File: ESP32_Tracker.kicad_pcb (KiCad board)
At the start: 4 copper layers, 45.5 x 75.5 mm, 73 parts, among them J1 USB_C_Receptacle_USB2.0_16P, J2 Conn_01x02_Socket, J3 Conn_01x07_Socket, J4 MSD-4-A, SW1 SW_Push, SW2 SW_Push, SW3 SW_Push, SW4 SW_Push, SW5 SW_Push, U1 USBLC6-2SC6, U2 ESP32-S3-MINI-1, U3 MP2667, U4 XC6220B331MR-G, U5 LIS2MDL, U6 SAM-M10Q

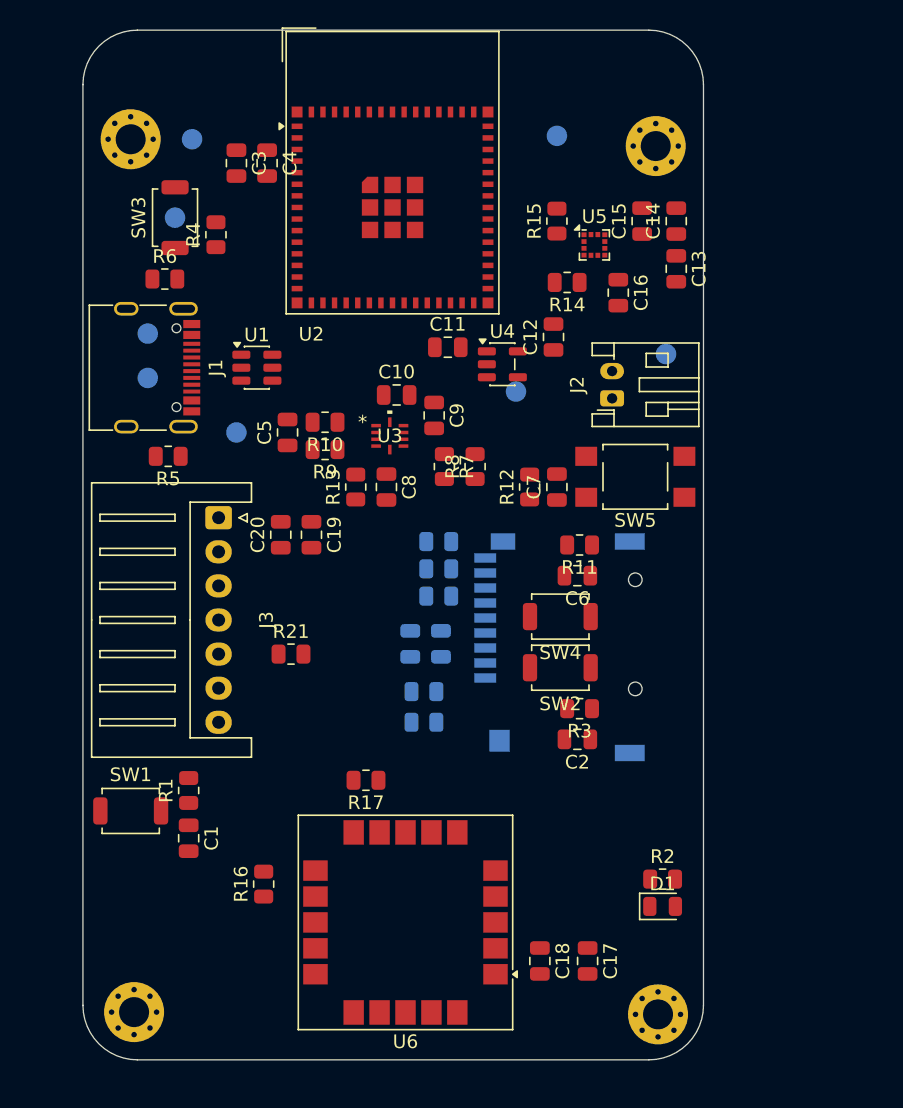
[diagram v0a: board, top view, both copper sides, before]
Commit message: Layout completed
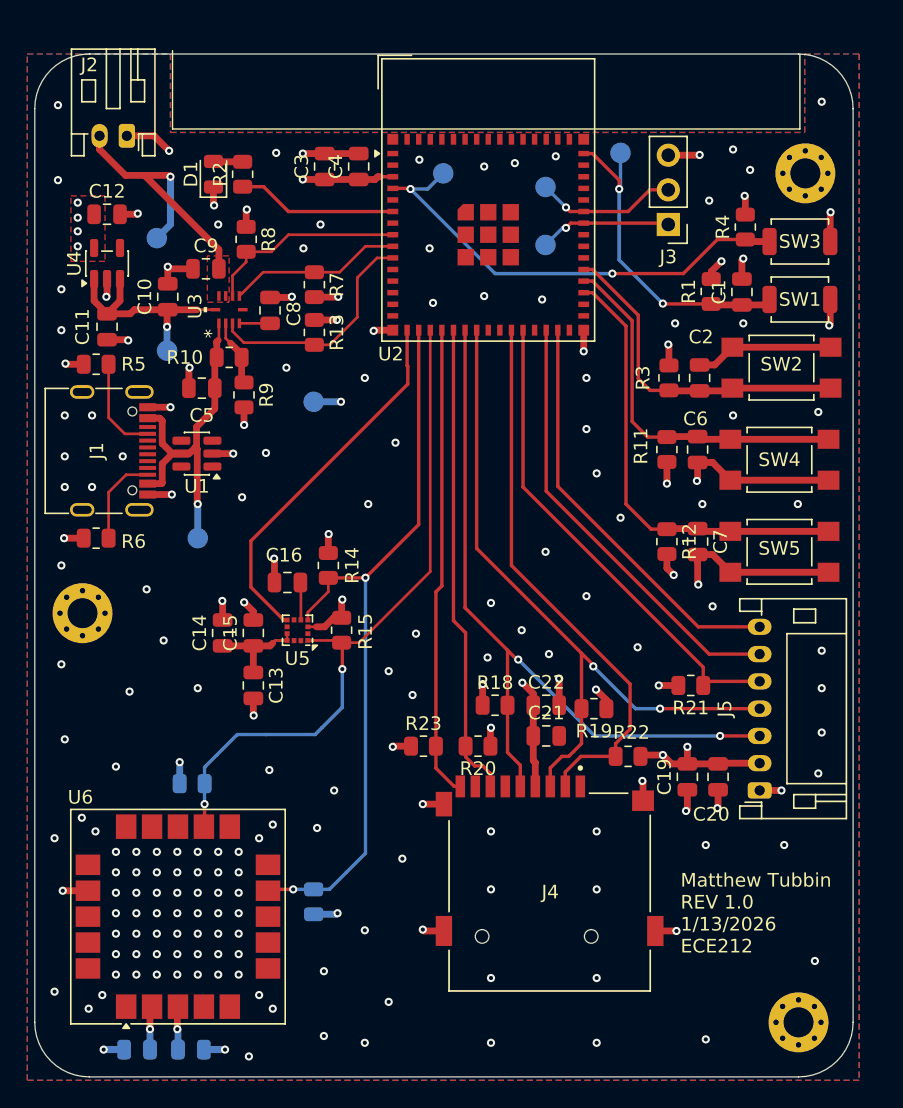
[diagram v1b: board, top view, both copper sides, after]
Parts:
- removed H4: MountingHole_Pad, MountingHole:MountingHole_2.2mm_M2_Pad_Via
- added J5: Conn_01x07_Socket, Connector_JST:JST_PH_S7B-PH-K_1x07_P2.00mm_Horizontal, F.Cu at (167.2, 116.0)
- C17: value 2.2u -> 10u; moved to B.Cu
- C18, R16, R17: moved to B.Cu
- C21, C22, J4, R18, R19, R20, R22, R23: moved to F.Cu
- J3: value Conn_01x07_Socket -> Conn_01x03; footprint Connector_JST:JST_XH_S7B-XH-A_1x07_P2.50mm_Horizontal -> Connector_PinHeader_2.54mm:PinHeader_1x03_P2.54mm_Vertical
- SW2, SW4: footprint Button_Switch_SMD:SW_SPST_TS-1088-xR020 -> Button_Switch_SMD:SW_SPST_TL3305C
- moved H2 81.2 mm to (170.1, 133.0)
- moved D1 63.0 mm to (127.2, 70.8), turned to 90 degrees
- moved SW1 61.8 mm to (170.2, 80.0), turned to 180 degrees
- moved R2 60.2 mm to (129.3, 70.8), turned to 90 degrees
- moved C1 57.0 mm to (165.9, 79.5), turned to 90 degrees
- moved R1 53.0 mm to (163.7, 79.4)
- moved SW3 45.8 mm to (170.2, 75.8), turned to 0 degrees
- moved C14 44.9 mm to (127.8, 104.5)
- moved C13 43.5 mm to (130.1, 108.3)
- moved C15 41.5 mm to (130.1, 104.5)
- moved J2 40.5 mm to (120.8, 68.0), turned to 180 degrees
- moved J3 39.4 mm to (160.5, 74.5), turned to 180 degrees
- moved R4 38.8 mm to (166.2, 74.7)
- moved TP6 38.3 mm to (123.0, 75.5)
- moved C20 36.6 mm to (164.2, 115.0), turned to -90 degrees
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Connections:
- net Net-(J2-Pin_2) renamed +BATT
- C2 pad 1: Net-(U2-IO18) -> /MCU/PWR/SW_TOGGLE
- C6 pad 1: Net-(U2-IO42) -> /MCU/PWR/SW_PWR
- C7 pad 1: Net-(U2-IO21) -> /MCU/PWR/SW_LOG
- J1 pad A6: Net-(J1-D+-PadA6) -> unconnected-(J1-D+-PadA6)
- J1 pad A7: Net-(J1-D--PadA7) -> unconnected-(J1-D--PadA7)
- J1 pad B6: Net-(J1-D+-PadA6) -> unconnected-(J1-D+-PadB6)
- J1 pad B7: Net-(J1-D--PadA7) -> unconnected-(J1-D--PadB7)
- J3 pad 1: GND -> /MCU/PWR/TX
- J3 pad 2: +3.3V -> /MCU/PWR/RX
- J3 pad 3: /MCU/PWR/OLED/SD_SCK -> GND
- R11 pad 1: Net-(U2-IO42) -> /MCU/PWR/SW_PWR
- R12 pad 1: Net-(U2-IO21) -> /MCU/PWR/SW_LOG
- R13 pad 2: /MCU/PWR/INT -> /MCU/PWR/BATT_INT
- R2 pad 1: Net-(U2-IO8) -> Net-(U2-IO2)
- R3 pad 1: Net-(U2-IO18) -> /MCU/PWR/SW_TOGGLE
- SW2 pad 1: Net-(U2-IO18) -> GND
- SW2 pad 2: GND -> /MCU/PWR/SW_TOGGLE
- SW4 pad 1: Net-(U2-IO42) -> /MCU/PWR/SW_PWR
- SW5 pad 1: Net-(U2-IO21) -> /MCU/PWR/SW_LOG
- TP2 pad 1: Net-(J1-D--PadA7) -> /MCU/PWR/TX
- TP3 pad 1: Net-(J1-D+-PadA6) -> /MCU/PWR/RX
- U1 pad 1: Net-(J1-D--PadA7) -> unconnected-(U1-I/O1-Pad1)
- U1 pad 3: Net-(J1-D+-PadA6) -> unconnected-(U1-I/O2-Pad3)
- U1 pad 4: /MCU/PWR/USB_P -> unconnected-(U1-I/O2-Pad4)
- U1 pad 6: /MCU/PWR/USB_N -> unconnected-(U1-I/O1-Pad6)
- U2 pad 10: /MCU/PWR/GPS/MAG_CLK -> /MCU/PWR/BATT_INT
- U2 pad 11: /MCU/PWR/OLED_CS -> unconnected-(U2-IO7-Pad11)
- U2 pad 12: Net-(U2-IO8) -> unconnected-(U2-IO8-Pad12)
- U2 pad 13: /MCU/PWR/SD_DETECT -> unconnected-(U2-IO9-Pad13)
- U2 pad 14: /MCU/PWR/SD_CS -> unconnected-(U2-IO10-Pad14)
- U2 pad 15: /MCU/PWR/OLED/SD_MOSI -> unconnected-(U2-IO11-Pad15)
- U2 pad 16: /MCU/PWR/OLED/SD_SCK -> /MCU/PWR/MAG_INT
- U2 pad 17: /MCU/PWR/SD_MISO -> /MCU/PWR/GPS/MAG_DATA
- U2 pad 18: unconnected-(U2-IO14-Pad18) -> /MCU/PWR/GPS/MAG_CLK
- U2 pad 19: unconnected-(U2-IO15-Pad19) -> /MCU/PWR/SD_DETECT
- U2 pad 20: /MCU/PWR/MAG_INT -> /MCU/PWR/SD_MISO
- U2 pad 21: unconnected-(U2-IO17-Pad21) -> /MCU/PWR/OLED/SD_SCK
- U2 pad 22: Net-(U2-IO18) -> /MCU/PWR/OLED/SD_MOSI
- U2 pad 23: /MCU/PWR/USB_N -> unconnected-(U2-USB_D--Pad23)
- U2 pad 24: /MCU/PWR/USB_P -> unconnected-(U2-USB_D+-Pad24)
- U2 pad 25: Net-(U2-IO21) -> /MCU/PWR/SD_CS
- U2 pad 26: /MCU/PWR/OLED_RST -> /MCU/PWR/OLED_CS
- U2 pad 28: unconnected-(U2-IO33-Pad28) -> /MCU/PWR/OLED_DC
- U2 pad 29: /MCU/PWR/BATT_DATA -> /MCU/PWR/OLED_RST
- U2 pad 31: /MCU/PWR/BATT_CLK -> unconnected-(U2-IO35-Pad31)
- U2 pad 33: unconnected-(U2-IO37-Pad33) -> /MCU/PWR/SW_LOG
- U2 pad 34: unconnected-(U2-IO38-Pad34) -> /MCU/PWR/SW_PWR
- U2 pad 35: unconnected-(U2-IO39-Pad35) -> /MCU/PWR/SW_TOGGLE
- U2 pad 38: Net-(U2-IO42) -> unconnected-(U2-IO42-Pad38)
- U2 pad 39: unconnected-(U2-TXD0-Pad39) -> /MCU/PWR/TX
- U2 pad 40: unconnected-(U2-RXD0-Pad40) -> /MCU/PWR/RX
- U2 pad 6: unconnected-(U2-IO2-Pad6) -> Net-(U2-IO2)
- U2 pad 8: /MCU/PWR/OLED_DC -> /MCU/PWR/BATT_DATA
- U2 pad 9: /MCU/PWR/GPS/MAG_DATA -> /MCU/PWR/BATT_CLK
- U3 pad 3: /MCU/PWR/INT -> /MCU/PWR/BATT_INT
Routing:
- net GND: track 0.00 -> 95.8 mm, vias 0 -> 183
- net +3.3V: track 0.00 -> 71.5 mm, vias 0 -> 29
- net /MCU/PWR/OLED/SD_SCK: track 0.00 -> 56.2 mm, vias 0 -> 2
- net /MCU/PWR/GPS/MAG_DATA: track 0.00 -> 54.7 mm, vias 0 -> 2
- net /MCU/PWR/OLED/SD_MOSI: track 0.00 -> 52.7 mm, vias 0 -> 2
- net /MCU/PWR/GPS/MAG_CLK: track 0.00 -> 50.0 mm, vias 0 -> 2
- net /MCU/PWR/SD_CS: track 0.00 -> 40.5 mm
- net /MCU/PWR/OLED_CS: track 0.00 -> 35.8 mm
- net /MCU/PWR/SD_MISO: track 0.00 -> 34.9 mm
- net /MCU/PWR/SD_DETECT: track 0.00 -> 34.6 mm
- net Net-(U2-IO0): track 0.00 -> 34.2 mm, vias 0 -> 2
- net /MCU/PWR/SW_LOG: track 0.00 -> 32.9 mm
- net /MCU/PWR/OLED_DC: track 0.00 -> 32.4 mm
- net /MCU/PWR/OLED_RST: track 0.00 -> 30.5 mm
- net /MCU/PWR/MAG_INT: track 0.00 -> 27.3 mm
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- added copper zone on F.Cu, net +3.3V
- added copper zone on In2.Cu, net +3.3V
- added copper zone on F.Cu, net +BATT
- added copper zone on B.Cu, net GND
- added copper zone on F.Cu, net GND
- added copper zone on In1.Cu, net GND
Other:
- board size 45.5 x 75.5 mm -> 60 x 75 mm
- board text added: "Matthew Tubbin REV 1.0 1/13/2026 ECE212"
